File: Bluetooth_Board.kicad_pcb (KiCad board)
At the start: 4 copper layers, 65 x 65 mm, 60 parts, among them IC1 STM32WB55CGU6, J1 5V Power Pins, J10 LPUART1_Header, J11 3V3 Power Pins, J13 3V3 Power Source Jumpers, J14 Debug_Pins, J15 USART1_Header, J19 Power Select Jumpers, J2 SMA PCB END LAUNCH JACK ROUND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, J20 SPI1_Header, J3 User Button Jumper, J4 Coin Battery Jumper, J5 Power Pins, J6 USB_B_Micro, J7 Pin_Header, J8 BOOT0_Jumper, J9 I2C1_Header, U3 USBLC6-2SC6, Y3 Clock_ECS-327MVATX-7-CN-TR, Y4 ABM3B-32.000MHZ-8-R30-B1U-T

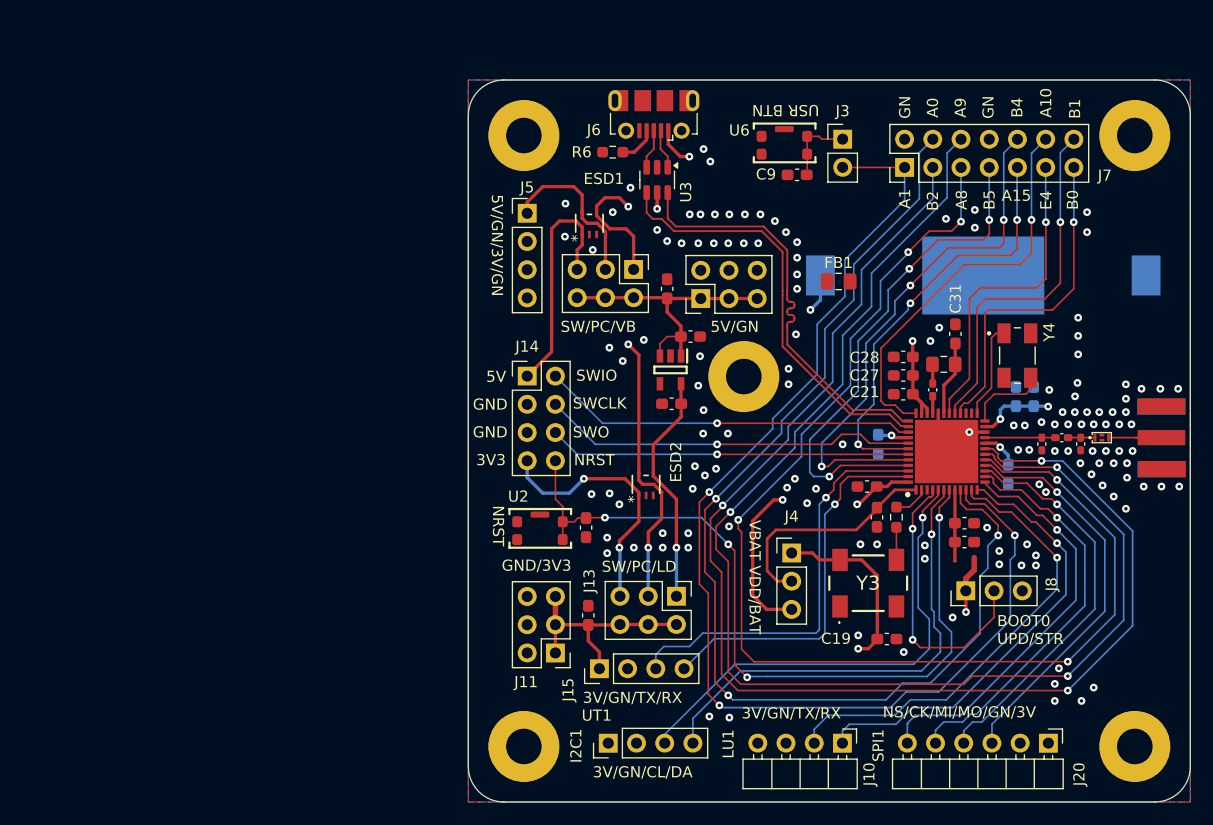
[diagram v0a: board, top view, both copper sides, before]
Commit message: update
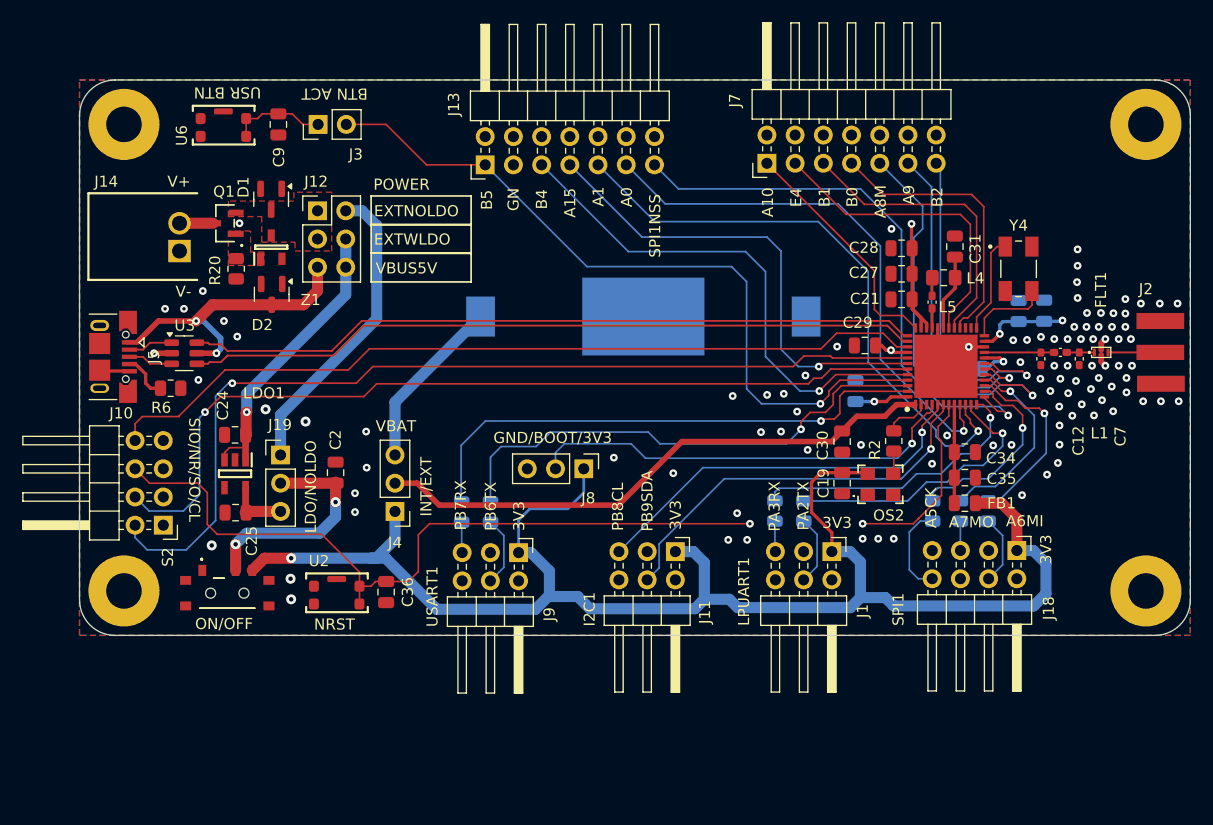
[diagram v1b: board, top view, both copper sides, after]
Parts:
- removed C23, C26: 4u7, Capacitor_SMD:C_0603_1608Metric_Pad1.08x0.95mm_HandSolder
- removed ESD1, ESD2: ESDALC6V1W5, Personal_Project:SOT323-5L_STM-L
- removed H6: MountingHole_Pad, MountingHole:MountingHole_3.2mm_M3_Pad
- removed J15: USART1_Header, Connector_PinHeader_2.54mm:PinHeader_1x04_P2.54mm_Vertical
- removed J17: ~, Personal_Project:SMA Clip Mount Adapter (bottom)
- removed J20: SPI1_Header, Connector_PinHeader_2.54mm:PinHeader_1x06_P2.54mm_Horizontal
- removed J6: USB_B_Micro, Connector_USB:USB_Micro-B_Molex-105017-0001
- removed Y3: Clock_ECS-327MVATX-7-CN-TR, Personal_Project:Clock_ECS327MVATX7CNTR
- added C2: 4u7, Capacitor_SMD:C_0805_2012Metric, F.Cu at (47.0, 57.4)
- added D1: BZX84C4V3LT1G, Package_TO_SOT_SMD:SOT-23, F.Cu at (41.2, 32.7)
- added D2: BZX84C6V2LT1G, Package_TO_SOT_SMD:SOT-23, F.Cu at (41.3, 41.3)
- added J12: Power_Selector_Jumper, Connector_PinHeader_2.54mm:PinHeader_2x03_P2.54mm_Vertical, F.Cu at (45.4, 33.8)
- added J18: SPI1_Headers, Connector_PinHeader_2.54mm:PinHeader_2x04_P2.54mm_Horizontal, F.Cu at (108.4, 64.4)
- added OS2: Oscillator_ECS-327MVATX-3-CN-TR, Personal_Project:Oscillator_ECS327MVATX3CNTR, F.Cu at (96.1, 58.4)
- added Q1: MOSFET_SI2333DDS-T1-BE3, Personal_Project:MOSFET_ SI2333DDS_SOT_DS-T1-BE3_VIS, F.Cu at (37.1, 34.9)
- added R1: 33R, Resistor_SMD:R_0805_2012Metric, B.Cu at (86.6, 60.8)
- added R20: 100k, Resistor_SMD:R_0805_2012Metric, F.Cu at (38.1, 39.0)
- added R3: 33R, Resistor_SMD:R_0805_2012Metric, B.Cu at (89.2, 60.8)
- added R4: 33R, Resistor_SMD:R_0805_2012Metric, B.Cu at (103.3, 60.8)
- added R5: 33R, Resistor_SMD:R_0805_2012Metric, B.Cu at (105.8, 60.8)
- added R7: 33R, Resistor_SMD:R_0805_2012Metric, B.Cu at (100.8, 60.8)
- added R8: 33R, Resistor_SMD:R_0805_2012Metric, B.Cu at (58.4, 60.9)
- added R9: 33R, Resistor_SMD:R_0805_2012Metric, B.Cu at (61.0, 60.9)
- added S2: Switch_WS-SLSU SMT Mini Slide, Personal_Project:Switch_WS-SLSU SMT Mini Slide, F.Cu at (37.3, 68.2)
- added Z1: Diode_BZX84C6V2-7-F, Personal_Project:Diode_BZX84C6V2_SOT96P240X110-3N, F.Cu at (41.3, 37.0)
- C19, C21, C22, C24, C25, C27, C28, C30, C31, C32, C33, C34, C35, C36, C9: footprint Capacitor_SMD:C_0603_1608Metric_Pad1.08x0.95mm_HandSolder -> Capacitor_SMD:C_0805_2012Metric
- C20: footprint Capacitor_SMD:C_0603_1608Metric_Pad1.08x0.95mm_HandSolder -> Capacitor_SMD:C_0805_2012Metric; moved to B.Cu
- C29: footprint Capacitor_SMD:C_0603_1608Metric_Pad1.08x0.95mm_HandSolder -> Capacitor_SMD:C_0805_2012Metric; moved to F.Cu
- FB1: footprint Capacitor_SMD:C_0805_2012Metric_Pad1.18x1.45mm_HandSolder -> Capacitor_SMD:C_0805_2012Metric
- J1: value 5V Power Pins -> LPUART1_Headers; footprint Connector_PinHeader_2.54mm:PinHeader_2x03_P2.54mm_Vertical -> Connector_PinHeader_2.54mm:PinHeader_2x03_P2.54mm_Horizontal
- J10: value LPUART1_Header -> Debug_Pins; footprint Connector_PinHeader_2.54mm:PinHeader_1x04_P2.54mm_Horizontal -> Connector_PinHeader_2.54mm:PinHeader_2x04_P2.54mm_Horizontal
- J11: value 3V3 Power Pins -> I2C1_Headers; footprint Connector_PinHeader_2.54mm:PinHeader_2x03_P2.54mm_Vertical -> Connector_PinHeader_2.54mm:PinHeader_2x03_P2.54mm_Horizontal
- J13: value 3V3 Power Source Jumpers -> General_Pin_Header; footprint Personal_Project:PinHeader_2x03_P2.54mm_Vertical_PINS -> Connector_PinHeader_2.54mm:PinHeader_2x07_P2.54mm_Horizontal
- J14: value Debug_Pins -> JST_XH_2.54_Plug; footprint Connector_PinHeader_2.54mm:PinHeader_2x04_P2.54mm_Vertical -> Personal_Project:Connector_Power2pin_SHDRRA2W80P0X250_1X2_740X1150X610P
- J19: value Power Select Jumpers -> 3V_Selection_Header; footprint Personal_Project:PinHeader_2x03_P2.54mm_Vertical_PINS -> Connector_PinHeader_2.54mm:PinHeader_1x03_P2.54mm_Vertical
- J5: value Power Pins -> USB_B_Micro; footprint Connector_PinHeader_2.54mm:PinHeader_1x04_P2.54mm_Vertical -> Connector_USB:USB_Micro-B_XKB_U254-051T-4BH83-F1S
- J7: value Pin_Header -> General_Pin_Header; footprint Connector_PinHeader_2.54mm:PinHeader_2x07_P2.54mm_Vertical -> Connector_PinHeader_2.54mm:PinHeader_2x07_P2.54mm_Horizontal
- J9: value I2C1_Header -> USART1_Headers; footprint Connector_PinHeader_2.54mm:PinHeader_1x04_P2.54mm_Vertical -> Connector_PinHeader_2.54mm:PinHeader_2x03_P2.54mm_Horizontal
- R2, R6: footprint Resistor_SMD:R_0603_1608Metric_Pad0.98x0.95mm_HandSolder -> Resistor_SMD:R_0805_2012Metric
- moved J10 64.2 mm to (31.5, 62.1), turned to 180 degrees
- moved U6 50.5 mm to (34.5, 27.6)
- moved J3 47.2 mm to (45.5, 26.0), turned to 90 degrees
- moved C9 46.9 mm to (41.9, 26.0), turned to 90 degrees
- moved U3 45.3 mm to (33.4, 46.6), turned to 0 degrees
- moved R6 45.1 mm to (32.2, 49.8), turned to 180 degrees
- moved J13 42.7 mm to (60.5, 29.6), turned to 90 degrees
- moved C24 41.9 mm to (38.0, 54.0), turned to 180 degrees
- moved C25 40.5 mm to (38.0, 61.0)
- moved LDO1 40.3 mm to (38.0, 57.5)
- moved J5 40.2 mm to (26.2, 46.9), turned to -90 degrees
- moved H4 38.6 mm to (28.0, 68.0)
- moved J8 36.1 mm to (69.4, 57.0), turned to -90 degrees
- moved H1 36.0 mm to (28.0, 26.0)
- moved J4 35.9 mm to (52.4, 60.8), turned to 180 degrees
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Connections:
- C24 pad 1: +5V -> /LDO_IN
- J1 pad 1: +5V -> +3.3V
- J1 pad 3: +5V -> GND
- J1 pad 4: GND -> Net-(J1-Pin_4)
- J1 pad 5: +5V -> Net-(J1-Pin_5)
- J10 pad 1: /PA3_LPUART1_RX -> GND
- J10 pad 2: /PA2_LPUART1_TX -> /PA14_SWCLK
- J10 pad 4: +3.3V -> /PB3_SWO
- J11 pad 3: +3.3V -> GND
- J11 pad 4: GND -> /PB9_I2C1_SDA
- J11 pad 5: +3.3V -> /PB8_I2C1_SCL
- J13 pad 1: /LD_OUT_3V3 -> /PB5
- J13 pad 2: /PC_3V3 -> GND
- J13 pad 3: /3V3_SW -> GND
- J13 pad 4: +3.3V -> GND
- J13 pad 5: +3.3V -> /PB4
- J13 pad 6: +3.3V -> GND
- J14 pad 1: /5V_SW -> GND
- J14 pad 2: /PA13_SWDIO -> /EXT_POWER+
- J19 pad 1: /VBUS -> /EXT_POWER+_NOLDO
- J19 pad 2: /PC_5V -> /POWER_3V3
- J19 pad 3: /5V_SW -> /LD_OUT_3V3
- J3 pad 2: /PA1 -> /PB5
- J5 pad 1: /PC_5V -> /VBUS_5V
- J5 pad 2: GND -> /USB_D2-
- J5 pad 3: /PC_3V3 -> /USB_D2+
- J5 pad 4: GND -> Net-(J5-ID)
- J7 pad 1: /PA1 -> /PA10
- J7 pad 10: /PB4 -> GND
- J7 pad 11: /PE4 -> /PA9
- J7 pad 12: /PA10 -> GND
- J7 pad 13: /PB0 -> /PB2
- J7 pad 14: /PB1 -> GND
- J7 pad 3: /PB2 -> /PE4
- J7 pad 4: /PA0 -> GND
- J7 pad 5: /PA8_MCO -> /PB1
- J7 pad 6: /PA9 -> GND
- J7 pad 7: /PB5 -> /PB0
- J7 pad 9: /PA15 -> /PA8_MCO
- J9 pad 3: /PB8_I2C1_SCL -> GND
- J9 pad 4: /PB9_I2C1_SDA -> Net-(J9-Pin_4)
- LDO1 pad 1: +5V -> /LDO_IN
- LDO1 pad 3: +5V -> /LDO_IN
- R6 pad 2: Net-(J6-ID) -> Net-(J5-ID)
- U3 pad 5: /VBUS -> /VBUS_5V
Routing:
- net /PA9: track 119.3 -> 30.2 mm, vias 3 -> 1
- net /PB2: track 119.5 -> 31.6 mm, vias 3 -> 1
- net /PA8_MCO: track 110.4 -> 37.8 mm, vias 5 -> 1
- net /PA1: track 106.4 -> 53.2 mm, vias 3 -> 1
- net /PA0: track 100.6 -> 48.8 mm, vias 3 -> 1
- net /PA14_SWCLK: track 34.0 -> 85.0 mm
- net /PB3_SWO: track 32.6 -> 79.4 mm
- net /PC_3V3: track 43.0 -> 0.00 mm, vias 2 -> 0
- net /PA13_SWDIO: track 33.9 -> 75.0 mm, vias 1 -> 0
- net /VBAT: track 20.8 -> 51.4 mm
- net +3.3V: track 231.1 -> 260.4 mm, vias 8 -> 7
- net /USB_D-: track 38.2 -> 66.0 mm
- net /USB_D+: track 38.3 -> 66.0 mm
- net /EXT_POWER+_NOLDO: track 0.00 -> 27.6 mm
- net /VBUS_5V: track 0.00 -> 27.4 mm, vias 0 -> 2
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- added copper zone on F.Cu, net /EXT_POWER+_PP
- added copper zone on F.Cu, net /MOSFET_GATE
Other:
- board size 65 x 65 mm -> 100 x 50 mm
- board text added: "A5CK"
- board text added: "A6MI"
- board text added: "A7MO"
- board text added: "A8M"
- board text added: "BTN ACT"
- board text added: "EXTNOLDO"
- board text added: "EXTWLDO"
- board text added: "GND/BOOT/3V3"
- board text added: "INT/EXT"
- board text added: "LDO/NOLDO"
- board text added: "LPUART1"
- board text added: "ON/OFF"
- board text added: "PA2TX"
- board text added: "PA3RX"
- board text added: "PB6TX"
- board text added: "PB7RX"
- board text added: "PB8CL"
- board text added: "PB9SDA"
- board text added: "POWER"
- board text added: "SIO/NR/SO/CL"
- board text added: "SPI1NSS"
- board text added: "USART1"
- board text added: "V+"
- board text added: "V-"
- board text added: "VBAT"
- board text added: "VBUS5V"
- board text removed: "3V/GN/CL/DA"
- board text removed: "3V/GN/TX/RX"
- board text removed: "5V"
- board text removed: "5V/GN"
- board text removed: "5V/GN/3V/GN"
- board text removed: "A8"
- board text removed: "BOOT0 UPD/STR"
- board text removed: "GND"
- board text removed: "GND/3V3"
- board text removed: "LU1"
- board text removed: "NS/CK/MI/MO/GN/3V"
- board text removed: "SW/PC/LD"
- board text removed: "SW/PC/VB"
- board text removed: "SWCLK"
- board text removed: "SWIO"
- board text removed: "SWO"
- board text removed: "UT1"
- board text removed: "VBAT VDD/BAT"
